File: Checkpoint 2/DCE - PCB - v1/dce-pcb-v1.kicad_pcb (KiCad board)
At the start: 2 copper layers, 52 parts, among them J1 Conn_01x06_Socket, J2 Conn_01x02_Socket, M1 2N7000, Q1 BC547B, Q2 BC547B, Q3 BC547B, Q4 BC557B, Q5 BC557B, Q6 BC547B, Q7 TIP41C, Q8 TIP42C, Q9 BC547B, U1 LM324

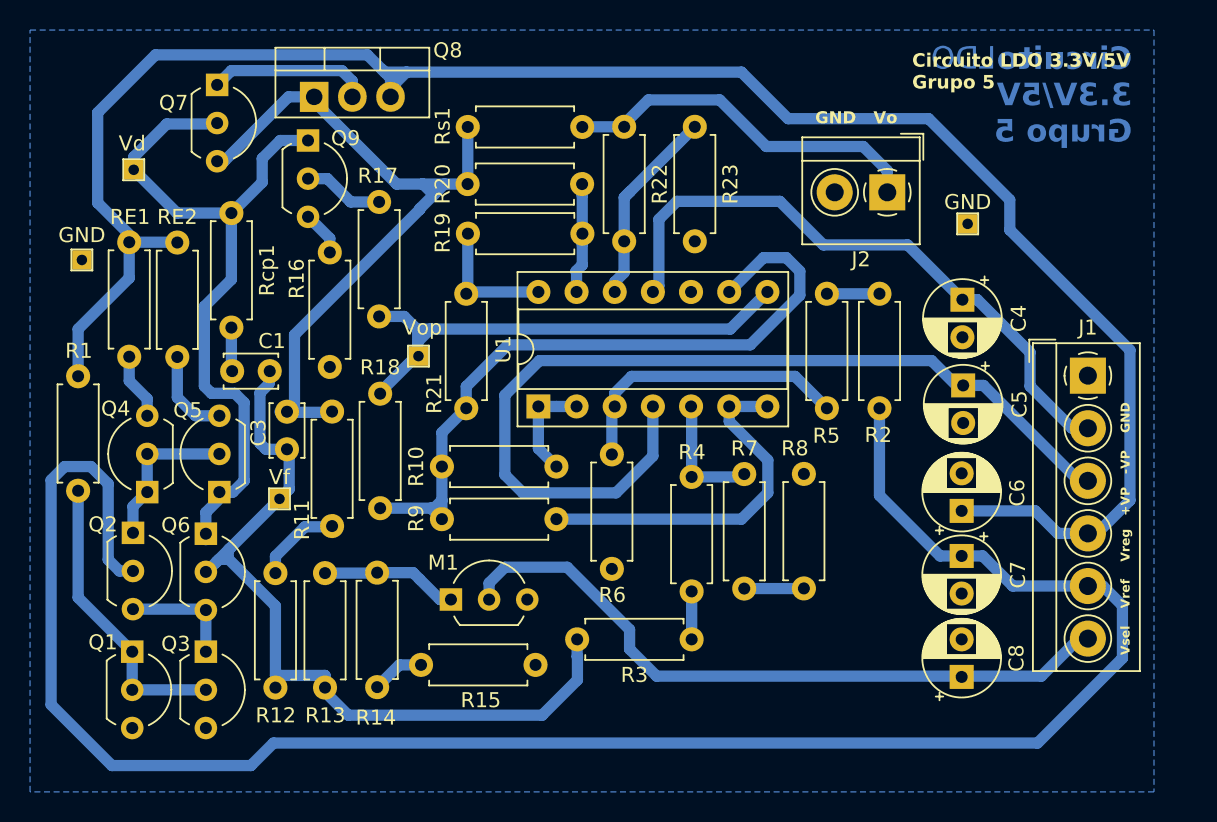
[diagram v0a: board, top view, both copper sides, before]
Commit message: actualizacion PCB
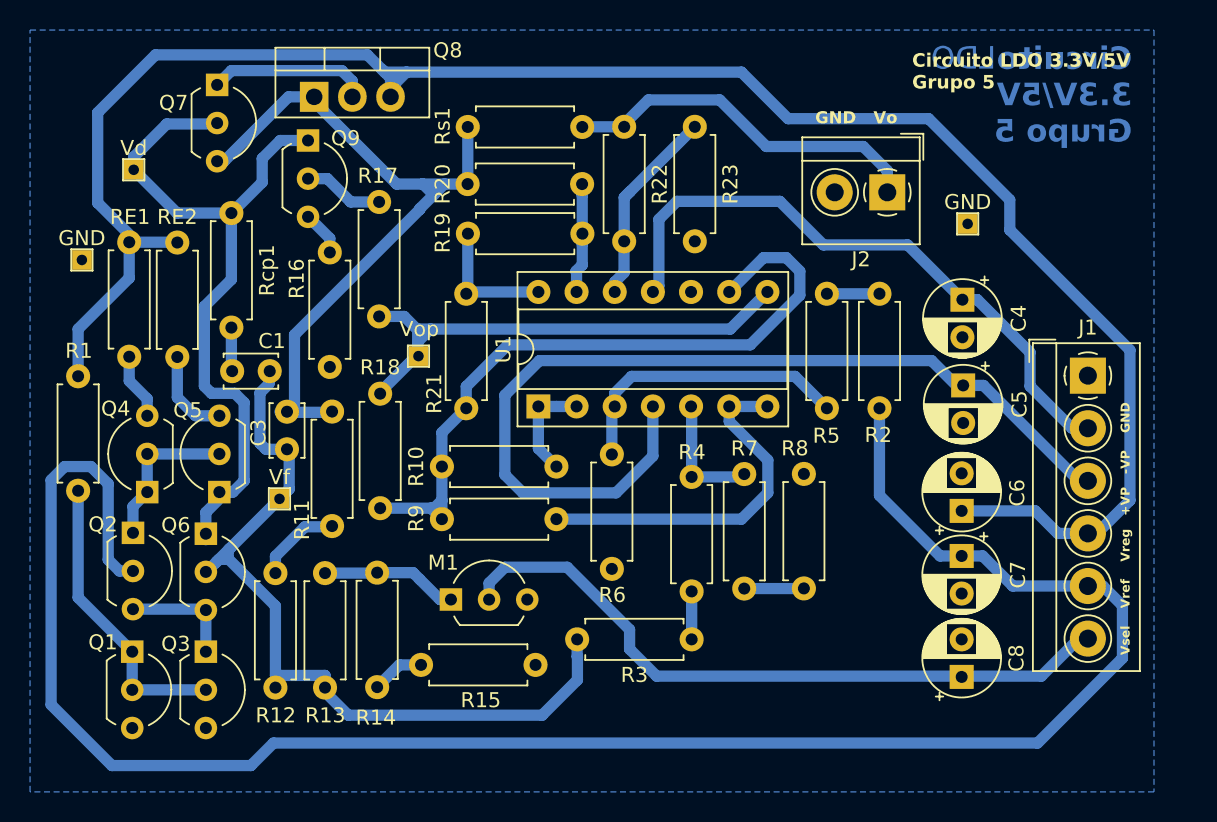
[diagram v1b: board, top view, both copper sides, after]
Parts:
- GND (x2), Vd, Vf, Vop: footprint TestPoint:TestPoint_THTPad_1.0x1.0mm_Drill0.5mm -> LDO_C2:TestPoint_THTPad_1.3x1.3mm_Drill0.7mm
- J1: footprint TerminalBlock_4Ucon:TerminalBlock_4Ucon_1x06_P3.50mm_Horizontal -> LDO_C2:TerminalBlock_4Ucon_1x06_P3.50mm_Horizontal
- J2: footprint TerminalBlock_4Ucon:TerminalBlock_4Ucon_1x02_P3.50mm_Horizontal -> LDO_C2:TerminalBlock_4Ucon_1x02_P3.50mm_Horizontal(3D)
- U1: footprint Package_DIP:DIP-14_W7.62mm_Socket -> LDO_C2:DIP-14_W7.62mm_Socket
